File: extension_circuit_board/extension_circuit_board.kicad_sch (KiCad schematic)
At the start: 7 parts, among them J1 AE_MRUSB_DIP, J2 Jetson_Nano_GPIO, J3 PiOLED 2x3, J4 FeatherWing_DCmotor, J5 Jetson Nano Power, J6 Motor Power, SW1 SW_SPDT

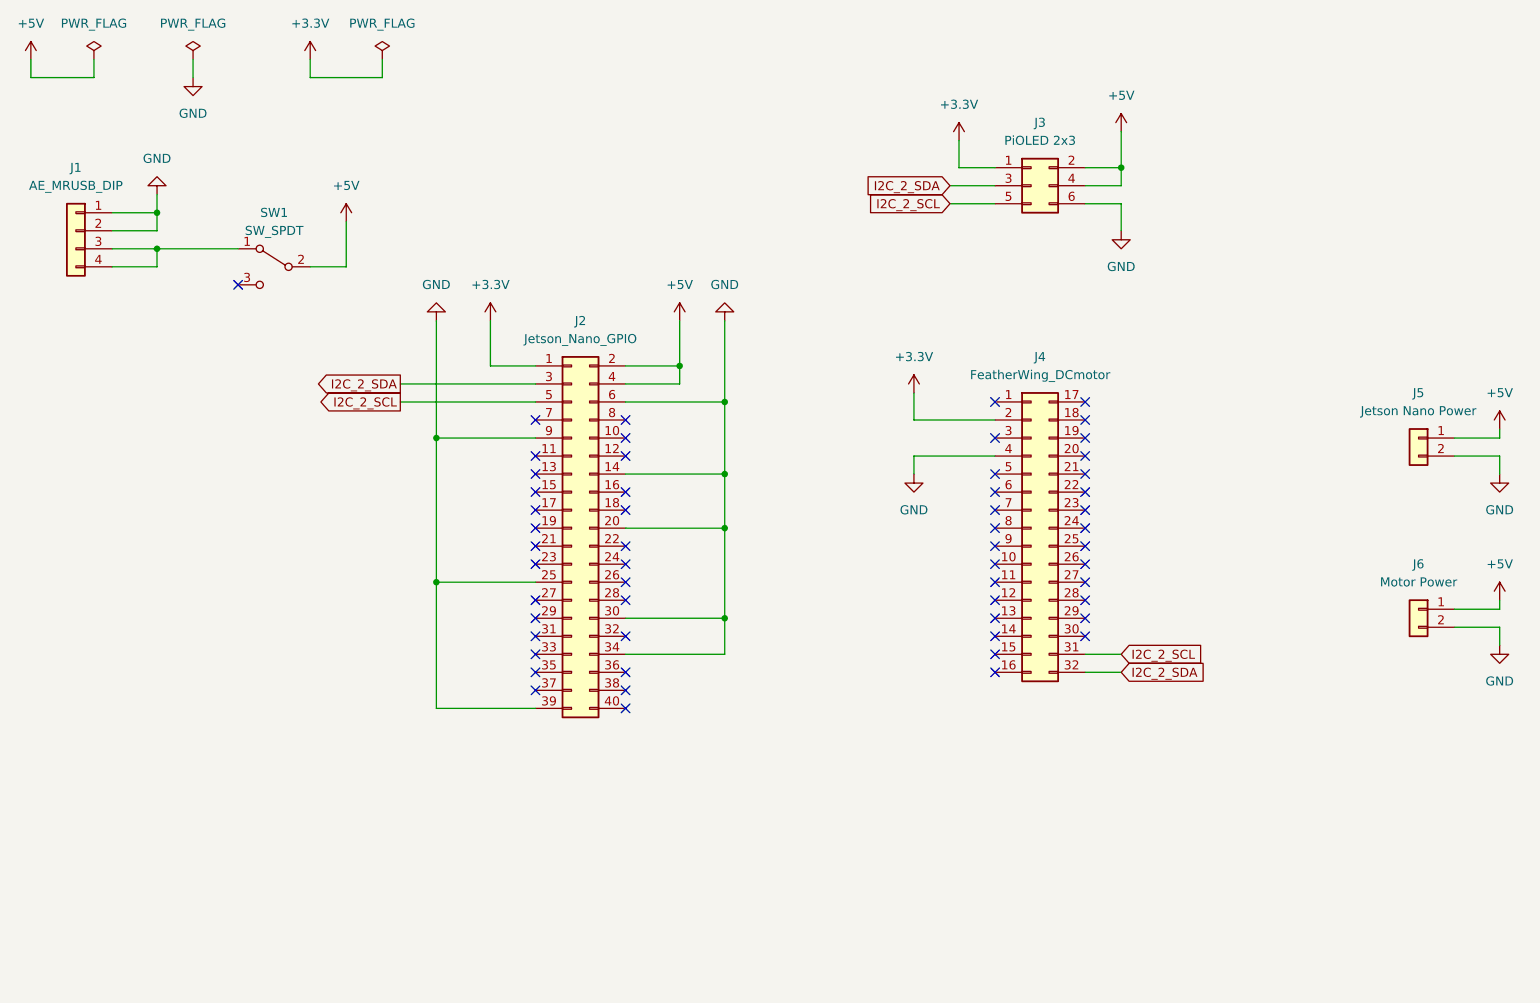
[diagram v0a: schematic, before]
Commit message: updated
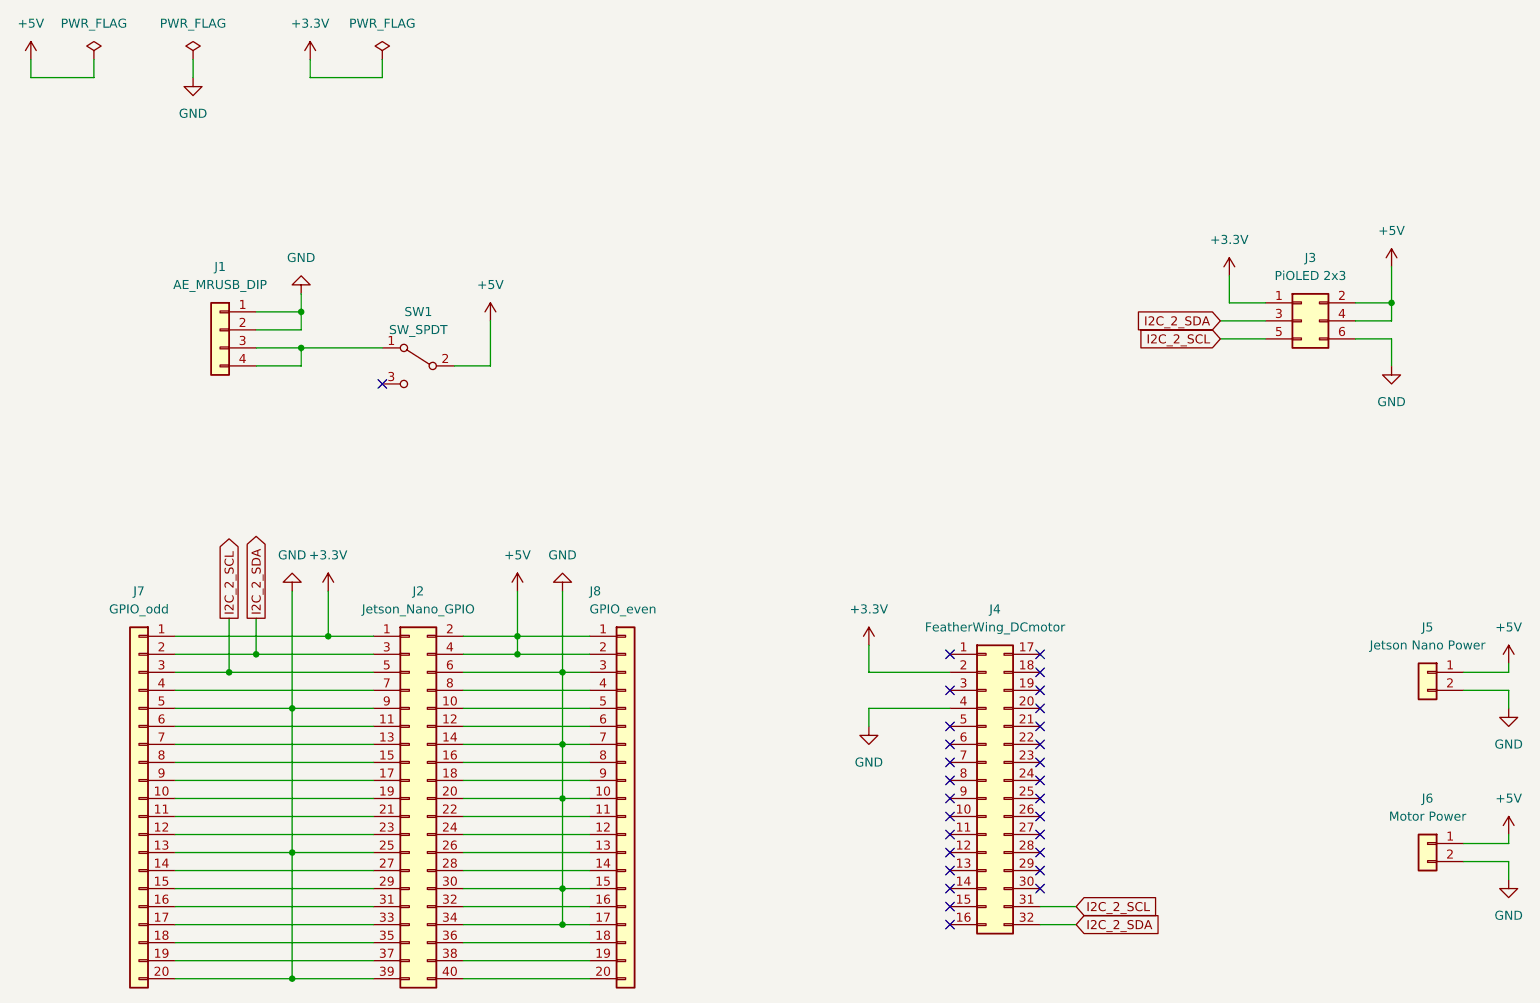
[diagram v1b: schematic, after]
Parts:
- added J7: GPIO_odd, Connector_PinHeader_2.54mm:PinHeader_1x20_P2.54mm_Vertical, symbol Connector_Generic:Conn_01x20
- added J8: GPIO_even, Connector_PinHeader_2.54mm:PinHeader_1x20_P2.54mm_Vertical, symbol Connector_Generic:Conn_01x20
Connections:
- net +3.3V: now also J7.1 (Pin_1)
- net +5V: now also J8.1 (Pin_1), J8.2 (Pin_2)
- net GND: now also J7.13 (Pin_13), J7.20 (Pin_20), J7.5 (Pin_5), J8.10 (Pin_10), J8.15 (Pin_15), J8.17 (Pin_17), J8.3 (Pin_3), J8.7 (Pin_7)
- net I2C_2_SCL: now also J7.3 (Pin_3)
- net I2C_2_SDA: now also J7.2 (Pin_2)
- net at J2.10 (Pin_10): now also J8.5 (Pin_5)
- net at J2.11 (Pin_11): now also J7.6 (Pin_6)
- net at J2.12 (Pin_12): now also J8.6 (Pin_6)
- net at J2.13 (Pin_13): now also J7.7 (Pin_7)
- net at J2.15 (Pin_15): now also J7.8 (Pin_8)
- net at J2.16 (Pin_16): now also J8.8 (Pin_8)
- net at J2.17 (Pin_17): now also J7.9 (Pin_9)
- net at J2.18 (Pin_18): now also J8.9 (Pin_9)
- net at J2.19 (Pin_19): now also J7.10 (Pin_10)
- net at J2.21 (Pin_21): now also J7.11 (Pin_11)
- net at J2.22 (Pin_22): now also J8.11 (Pin_11)
- net at J2.23 (Pin_23): now also J7.12 (Pin_12)
- net at J2.24 (Pin_24): now also J8.12 (Pin_12)
- net at J2.26 (Pin_26): now also J8.13 (Pin_13)
- net at J2.27 (Pin_27): now also J7.14 (Pin_14)
- net at J2.28 (Pin_28): now also J8.14 (Pin_14)
- net at J2.29 (Pin_29): now also J7.15 (Pin_15)
- net at J2.31 (Pin_31): now also J7.16 (Pin_16)
- net at J2.32 (Pin_32): now also J8.16 (Pin_16)
- net at J2.33 (Pin_33): now also J7.17 (Pin_17)
- net at J2.35 (Pin_35): now also J7.18 (Pin_18)
- net at J2.36 (Pin_36): now also J8.18 (Pin_18)
- net at J2.37 (Pin_37): now also J7.19 (Pin_19)
- net at J2.38 (Pin_38): now also J8.19 (Pin_19)
- net at J2.40 (Pin_40): now also J8.20 (Pin_20)
- net at J2.7 (Pin_7): now also J7.4 (Pin_4)
- net at J2.8 (Pin_8): now also J8.4 (Pin_4)
- no-connect marks 56 -> 29
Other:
- moved on the sheet: J1, J2, J3, J4, J5, J6, SW1
